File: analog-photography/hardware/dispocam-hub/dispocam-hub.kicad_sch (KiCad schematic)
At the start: 29 parts, among them J1 Conn_01x16, J2 Conn_01x12, M1 Motor_Servo_Pair, M2 Motor_Servo_Pair, M3 Motor_Servo_Pair, M4 Motor_Servo_Pair, SW1 Wind Limit, SW2 Wind Limit, SW3 Wind Limit, SW4 Wind Limit, SW5 Trigger, U1 TPS61023, U2 DS3231M

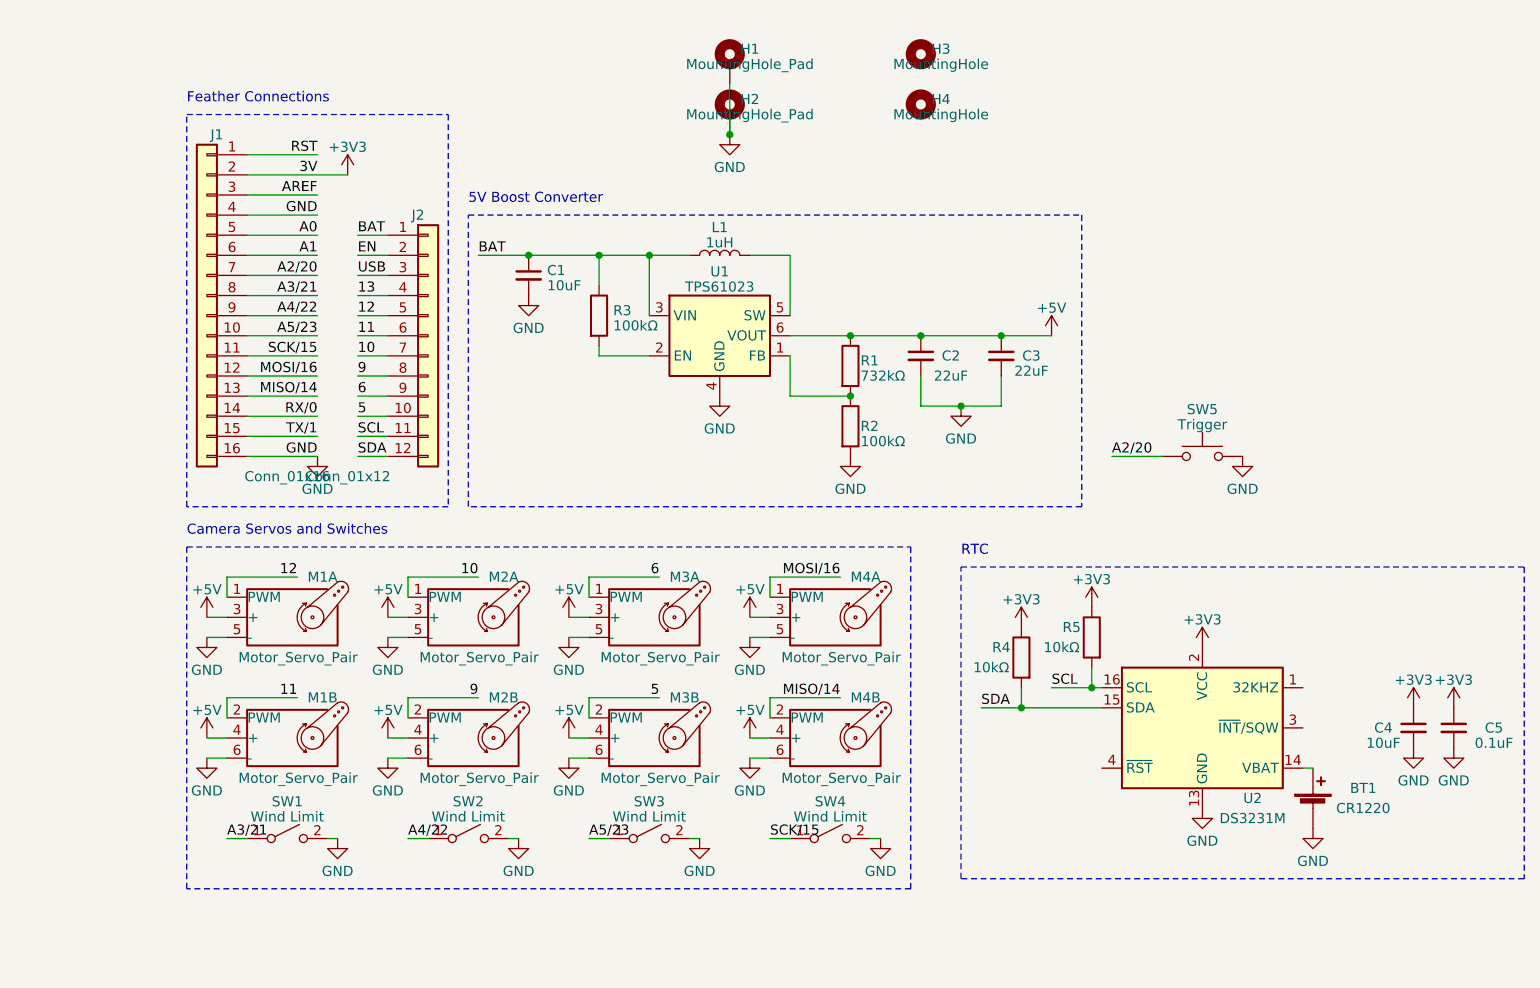
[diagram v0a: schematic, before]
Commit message: finalize PCB design, export gerbers, clean up schematic
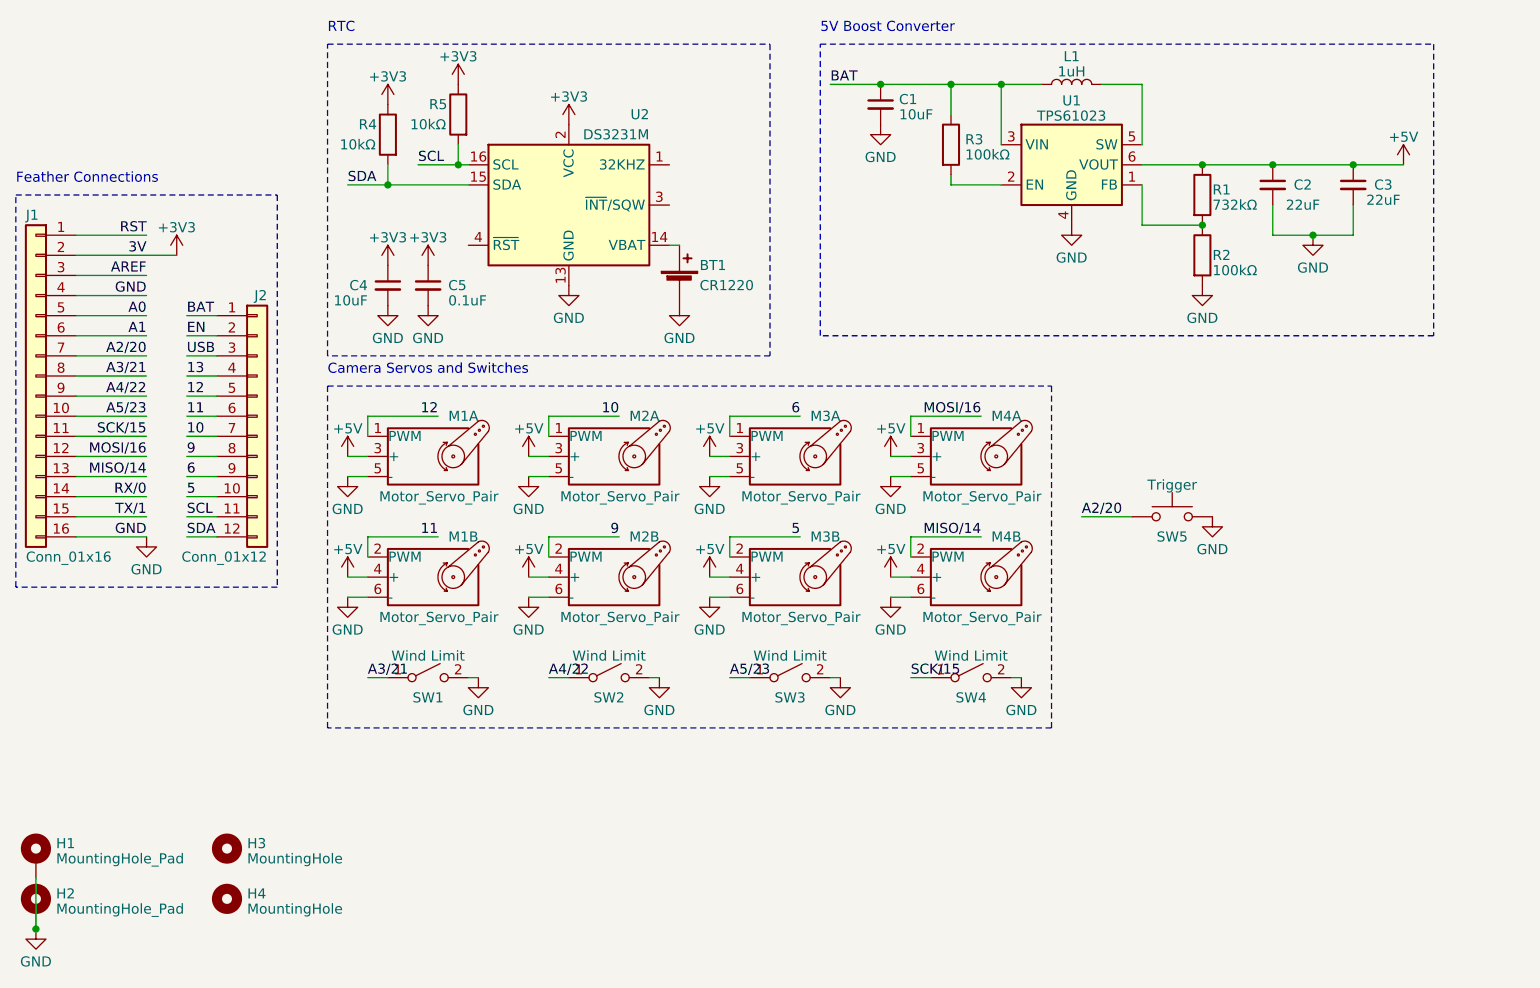
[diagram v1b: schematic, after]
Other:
- company: (none) -> Jacob Smilg
- title: (none) -> Dispocam Hub Featherwing
- moved on the sheet: BT1, C1, C2, C3, C4, C5, H1, H2, H3, H4, J1, J2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
